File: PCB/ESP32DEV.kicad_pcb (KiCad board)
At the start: 2 copper layers, 34.7 x 43.8 mm, 33 parts, among them J1 USB_C_Receptacle_USB2.0_16P, J2 Conn_01x18_Pin, J3 Conn_01x18_Pin, J5 Conn_01x04_Pin, J6 Conn_01x02_Pin, Q1 AO3401A, SW1 SW_Push, SW2 SW_Push, U2 AP63203WU, U5 ESP32-S3-WROOM-1

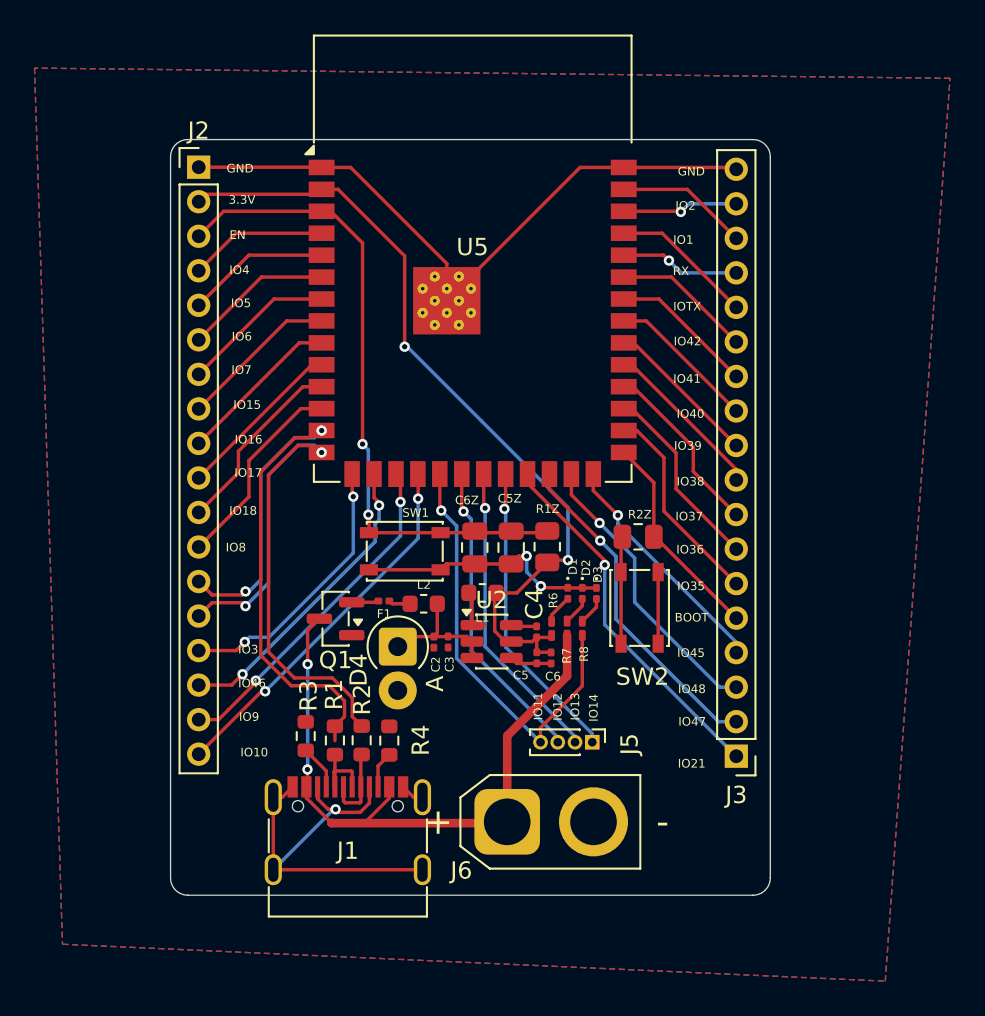
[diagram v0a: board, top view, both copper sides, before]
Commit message: Add files via upload
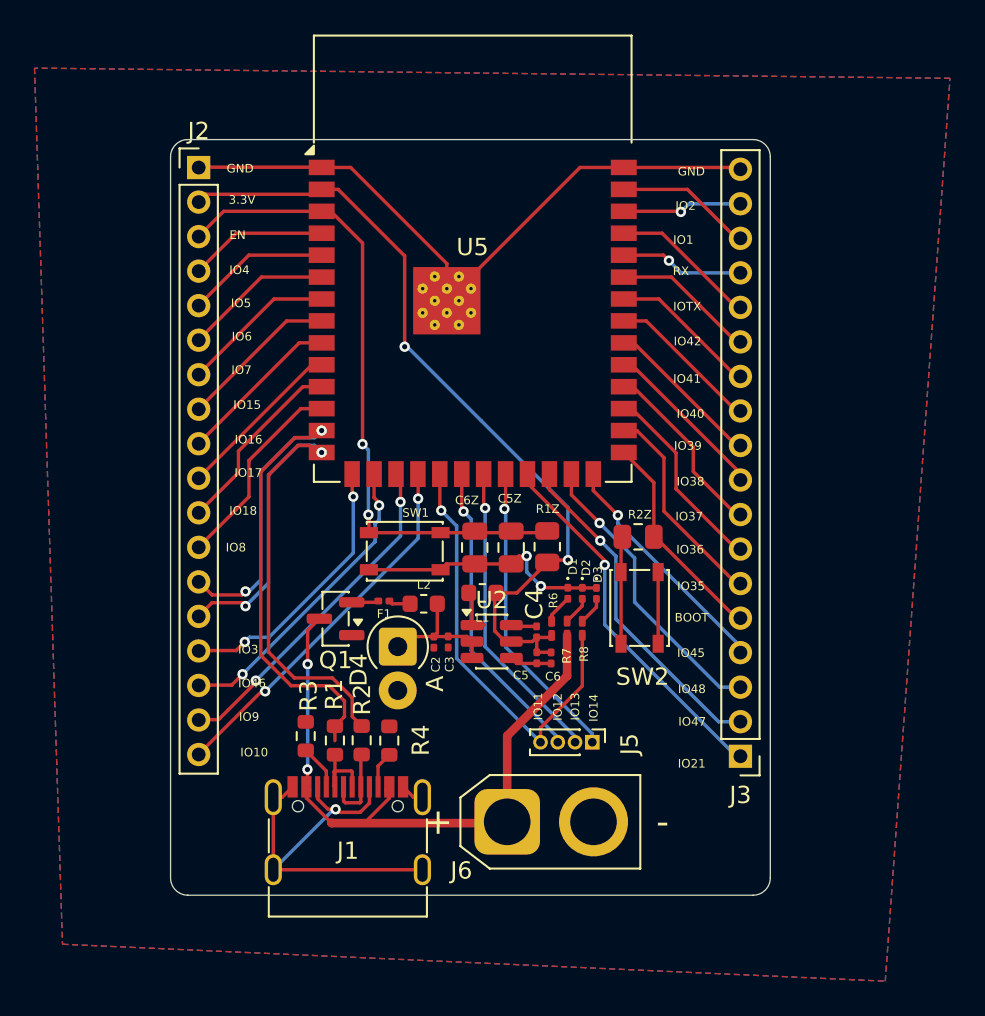
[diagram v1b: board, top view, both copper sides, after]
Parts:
- moved J3 0.24 mm to (142.2, 119.0)
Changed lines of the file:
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@@
 	(footprint "Connector_PinHeader_2.00mm:PinHeader_1x18_P2.00mm_Vertical"
 		(layer "F.Cu")
-		(at 142 119 180)
+		(at 142.24 119 180)
 		(descr "Through hole straight pin header, 1x18, 2.00mm pitch, single row")
 		(tags "Through hole pin header THT 1x18 2.00mm single row")
@@
 	(footprint "Connector_PinHeader_2.00mm:PinHeader_1x18_P2.00mm_Vertical"
 		(layer "F.Cu")
-		(at 110.86 84.88)
+		(at 110.86 84.9)
 		(descr "Through hole straight pin header, 1x18, 2.00mm pitch, single row")
 		(tags "Through hole pin header THT 1x18 2.00mm single row")
